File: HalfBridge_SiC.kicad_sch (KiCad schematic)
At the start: 3 parts, among them J4 Screw_Terminal_01x02

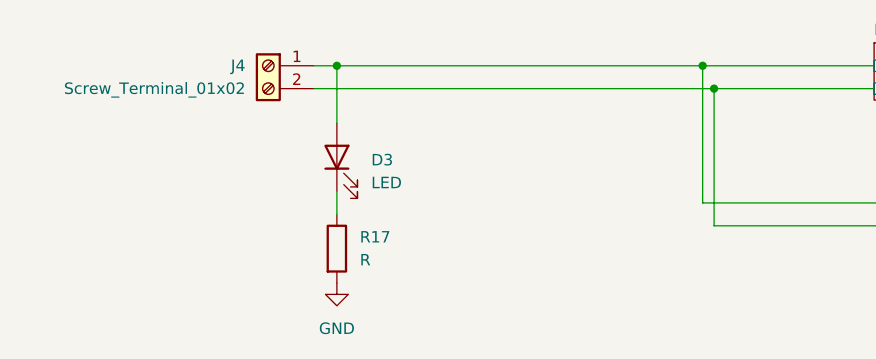
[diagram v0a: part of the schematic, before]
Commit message: position
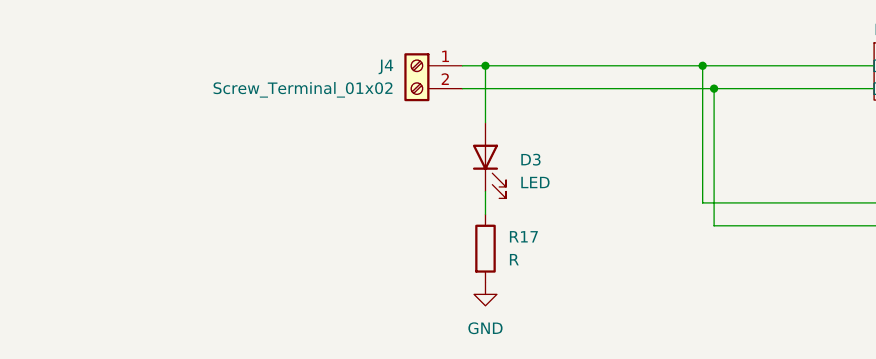
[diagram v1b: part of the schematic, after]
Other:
- moved on the sheet: D3, J4, R17
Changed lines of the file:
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@@
 	(paper "A4")
 	(junction
-		(at 27.94 95.25)
+		(at 44.45 95.25)
 		(diameter 0)
 		(color 0 0 0 0)
@@
 	(wire
 		(pts
-			(xy 25.4 95.25) (xy 27.94 95.25)
-		)
-		(stroke
-			(width 0)
-			(type default)
-		)
-	)
-	(wire
-		(pts
-			(xy 27.94 109.22) (xy 27.94 111.76)
+			(xy 41.91 95.25) (xy 44.45 95.25)
+		)
+		(stroke
+			(width 0)
+			(type default)
+		)
+	)
+	(wire
+		(pts
+			(xy 44.45 109.22) (xy 44.45 111.76)
 		)
 		(stroke
@@
 	(wire
 		(pts
-			(xy 27.94 95.25) (xy 68.58 95.25)
+			(xy 44.45 95.25) (xy 68.58 95.25)
 		)
 		(stroke
@@
 	(wire
 		(pts
-			(xy 25.4 97.79) (xy 69.85 97.79)
+			(xy 41.91 97.79) (xy 69.85 97.79)
 		)
 		(stroke
@@
 	(wire
 		(pts
-			(xy 27.94 95.25) (xy 27.94 101.6)
+			(xy 44.45 95.25) (xy 44.45 101.6)
 		)
 		(stroke
@@
 	(symbol
 		(lib_id "Connector:Screw_Terminal_01x02")
-		(at 20.32 95.25 0)
+		(at 36.83 95.25 0)
 		(mirror y)
 		(unit 1)
@@
 		(dnp no)
 		(property "Reference" "J4"
-			(at 17.78 95.2499 0)
+			(at 34.29 95.2499 0)
 			(effects
 				(font
@@
 		)
 		(property "Value" "Screw_Terminal_01x02"
-			(at 17.78 97.7899 0)
+			(at 34.29 97.7899 0)
 			(effects
 				(font
@@
 		)
 		(property "Footprint" "TerminalBlock_Phoenix:TerminalBlock_Phoenix_PT-1,5-2-3.5-H_1x02_P3.50mm_Horizontal"
-			(at 20.32 95.25 0)
+			(at 36.83 95.25 0)
 			(effects
 				(font
@@
 		)
 		(property "Datasheet" "~"
-			(at 20.32 95.25 0)
+			(at 36.83 95.25 0)
 			(effects
 				(font
@@
 		)
 		(property "Description" "Generic screw terminal, single row, 01x02, script generated (kicad-library-utils/schlib/autogen/connector/)"
-			(at 20.32 95.25 0)
+			(at 36.83 95.25 0)
 			(effects
 				(font
@@
 	(symbol
 		(lib_id "Device:R")
-		(at 27.94 115.57 0)
+		(at 44.45 115.57 0)
 		(unit 1)
 		(exclude_from_sim no)
@@
 		(fields_autoplaced yes)
 		(property "Reference" "R17"
-			(at 30.48 114.2999 0)
+			(at 46.99 114.2999 0)
 			(effects
 				(font
@@
 		)
 		(property "Value" "R"
-			(at 30.48 116.8399 0)
+			(at 46.99 116.8399 0)
 			(effects
 				(font
@@
 		)
 		(property "Footprint" "Resistor_SMD:R_0603_1608Metric"
-			(at 26.162 115.57 90)
+			(at 42.672 115.57 90)
 			(effects
 				(font
@@
 		)
 		(property "Datasheet" "~"
-			(at 27.94 115.57 0)
+			(at 44.45 115.57 0)
 			(effects
 				(font
@@
 		)
 		(property "Description" "Resistor"
-			(at 27.94 115.57 0)
+			(at 44.45 115.57 0)
 			(effects
 				(font
@@
 	(symbol
 		(lib_id "Device:LED")
-		(at 27.94 105.41 90)
+		(at 44.45 105.41 90)
 		(unit 1)
 		(exclude_from_sim no)
@@
 		(fields_autoplaced yes)
 		(property "Reference" "D3"
-			(at 31.75 105.7274 90)
+			(at 48.26 105.7274 90)
 			(effects
 				(font
@@
 		)
 		(property "Value" "LED"
-			(at 31.75 108.2674 90)
+			(at 48.26 108.2674 90)
 			(effects
 				(font
@@
 		)
 		(property "Footprint" "LED_SMD:LED_0603_1608Metric_Pad1.05x0.95mm_HandSolder"
-			(at 27.94 105.41 0)
+			(at 44.45 105.41 0)
 			(effects
 				(font
@@
 		)
 		(property "Datasheet" "~"
-			(at 27.94 105.41 0)
+			(at 44.45 105.41 0)
 			(effects
 				(font
@@
 		)
 		(property "Description" "Light emitting diode"
-			(at 27.94 105.41 0)
+			(at 44.45 105.41 0)
 			(effects
 				(font
@@
 	(symbol
 		(lib_id "power:GND")
-		(at 27.94 119.38 0)
+		(at 44.45 119.38 0)
 		(unit 1)
 		(exclude_from_sim no)
@@
 		(fields_autoplaced yes)
 		(property "Reference" "#PWR01"
-			(at 27.94 125.73 0)
+			(at 44.45 125.73 0)
 			(effects
 				(font
@@
 		)
 		(property "Value" "GND"
-			(at 27.94 124.46 0)
+			(at 44.45 124.46 0)
 			(effects
 				(font
@@
 		)
 		(property "Footprint" ""
-			(at 27.94 119.38 0)
+			(at 44.45 119.38 0)
 			(effects
 				(font
@@
 		)
 		(property "Datasheet" ""
-			(at 27.94 119.38 0)
+			(at 44.45 119.38 0)
 			(effects
 				(font
@@
 		)
 		(property "Description" "Power symbol creates a global label with name \"GND\" , ground"
-			(at 27.94 119.38 0)
-			(effects
-				(font
+			(at 44.45 119.38 0)
+			(effects
+				(font

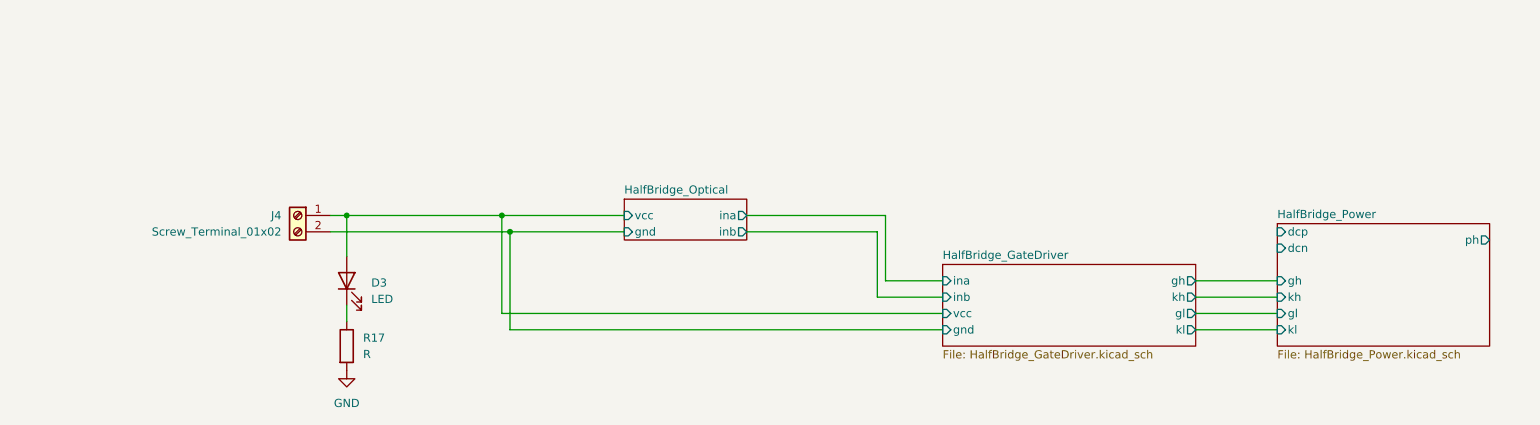
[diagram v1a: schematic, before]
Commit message: diff rx
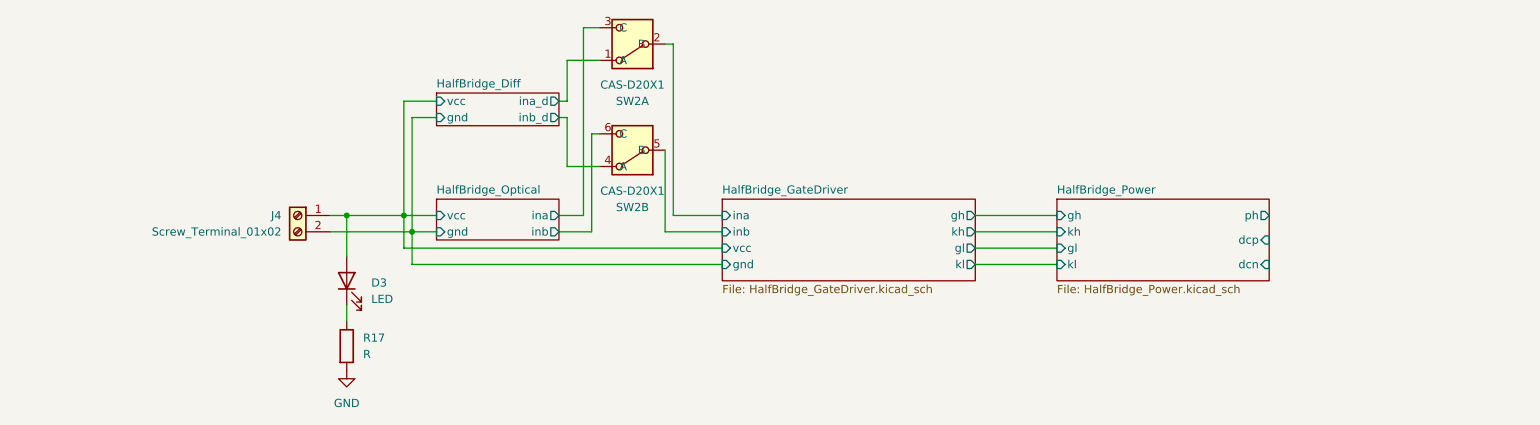
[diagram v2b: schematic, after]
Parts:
- added SW2: CAS-D20X1, My_Button_Switch_SMD:Nidec_Copal_CAS-D20A1, symbol My_Switch:CAS-D20X1
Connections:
- net HalfBridge_GateDriver/ina: now also SW2.2 (B)
- net HalfBridge_GateDriver/inb: now also SW2.5 (B)
- net HalfBridge_GateDriver/gnd renamed HalfBridge_Diff/gnd
- net HalfBridge_GateDriver/vcc renamed HalfBridge_Diff/vcc
- new net HalfBridge_Diff/ina_d: SW2.1 (A)
- new net HalfBridge_Diff/inb_d: SW2.4 (A)
- new net HalfBridge_Optical/ina: SW2.3 (C)
- new net HalfBridge_Optical/inb: SW2.6 (C)
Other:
- added sheet HalfBridge_Diff (HalfBridge_Diff.kicad_sch)
